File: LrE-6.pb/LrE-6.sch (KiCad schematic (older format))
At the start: 115 parts, among them J1 USB_B_Micro, J2 SM06B-SRSS-TB, J3 LP_Header_02x03, J4 LP_Header_01x02, Q1 2N7002, Q11 2N7002, SW1 SW_Push_45deg, SW10 SW_Push_45deg, SW11 Rotary_Encoder_Switch, SW12 Rotary_Encoder_Switch, SW13 Rotary_Encoder_Switch, SW14 Rotary_Encoder_Switch, SW15 Rotary_Encoder_Switch, SW16 Rotary_Encoder_Switch, SW2 SW_Push_45deg, SW3 SW_Push_45deg, SW4 SW_Push_45deg, SW5 SW_Push_45deg, SW6 SW_Push_45deg, SW7 SW_Push_45deg, SW8 SW_Push_45deg, SW9 SW_Push_45deg, U1 STM32F072C8Tx, U2 ESP-WROOM-02, U3 AQM0802-FLW-GBW, U4 SPX3819M5-L3-3TR

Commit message: 0.27-5
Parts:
- removed C20: 0.1u, Capacitor_SMD:C_0805_2012Metric, symbol LrE-6-rescue:C-Device
- removed C28: 10u, Capacitor_SMD:C_0805_2012Metric, symbol LrE-6-rescue:C-Device
- removed J3: LP_Header_02x03, Connector_PinHeader_2.54mm:PinHeader_2x03_P2.54mm_Vertical, symbol LrE-6-rescue:Conn_02x03_Odd_Even-Connector_Generic
- removed J4: LP_Header_01x02, Connector_PinHeader_2.54mm:PinHeader_1x02_P2.54mm_Vertical, symbol LrE-6-rescue:Conn_02x01-Connector_Generic
- removed R33: 10K, Resistor_SMD:R_0805_2012Metric, symbol LrE-6-rescue:R-Device
- removed R34: 100, Resistor_SMD:R_0805_2012Metric, symbol LrE-6-rescue:R-Device
- removed R36, R37: 10K, Resistor_SMD:R_0805_2012Metric, symbol Device:R
- removed U2: ESP-WROOM-02, RF_Module:ESP-WROOM-02, symbol LrE-6-rescue:ESP-WROOM-02-RF_Module
- C30, C31, C32, C33, C34, C35, C36: symbol Device:C -> LrE-6-rescue:C-Device
- Q1: symbol Transistor_FET:2N7002 -> LrE-6-rescue:2N7002-Transistor_FET
- R21: symbol Device:R -> LrE-6-rescue:R-Device
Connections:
- net labels removed: ENC6-A, ENC6-B, STM_RX, STM_TX, WL_0, WL_EN, WL_RST, WL_RXD, WL_TXD
- wire segments 462 -> 419
- no-connect marks 19 -> 14
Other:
- note added: "R2.1\n"
- note removed: "FT234X"
- note removed: "GND"
- note removed: "N.C.(5V)"
- note removed: "R2.02"
- note removed: "RXD"
- note removed: "TXD"
- moved on the sheet: Q1, R21

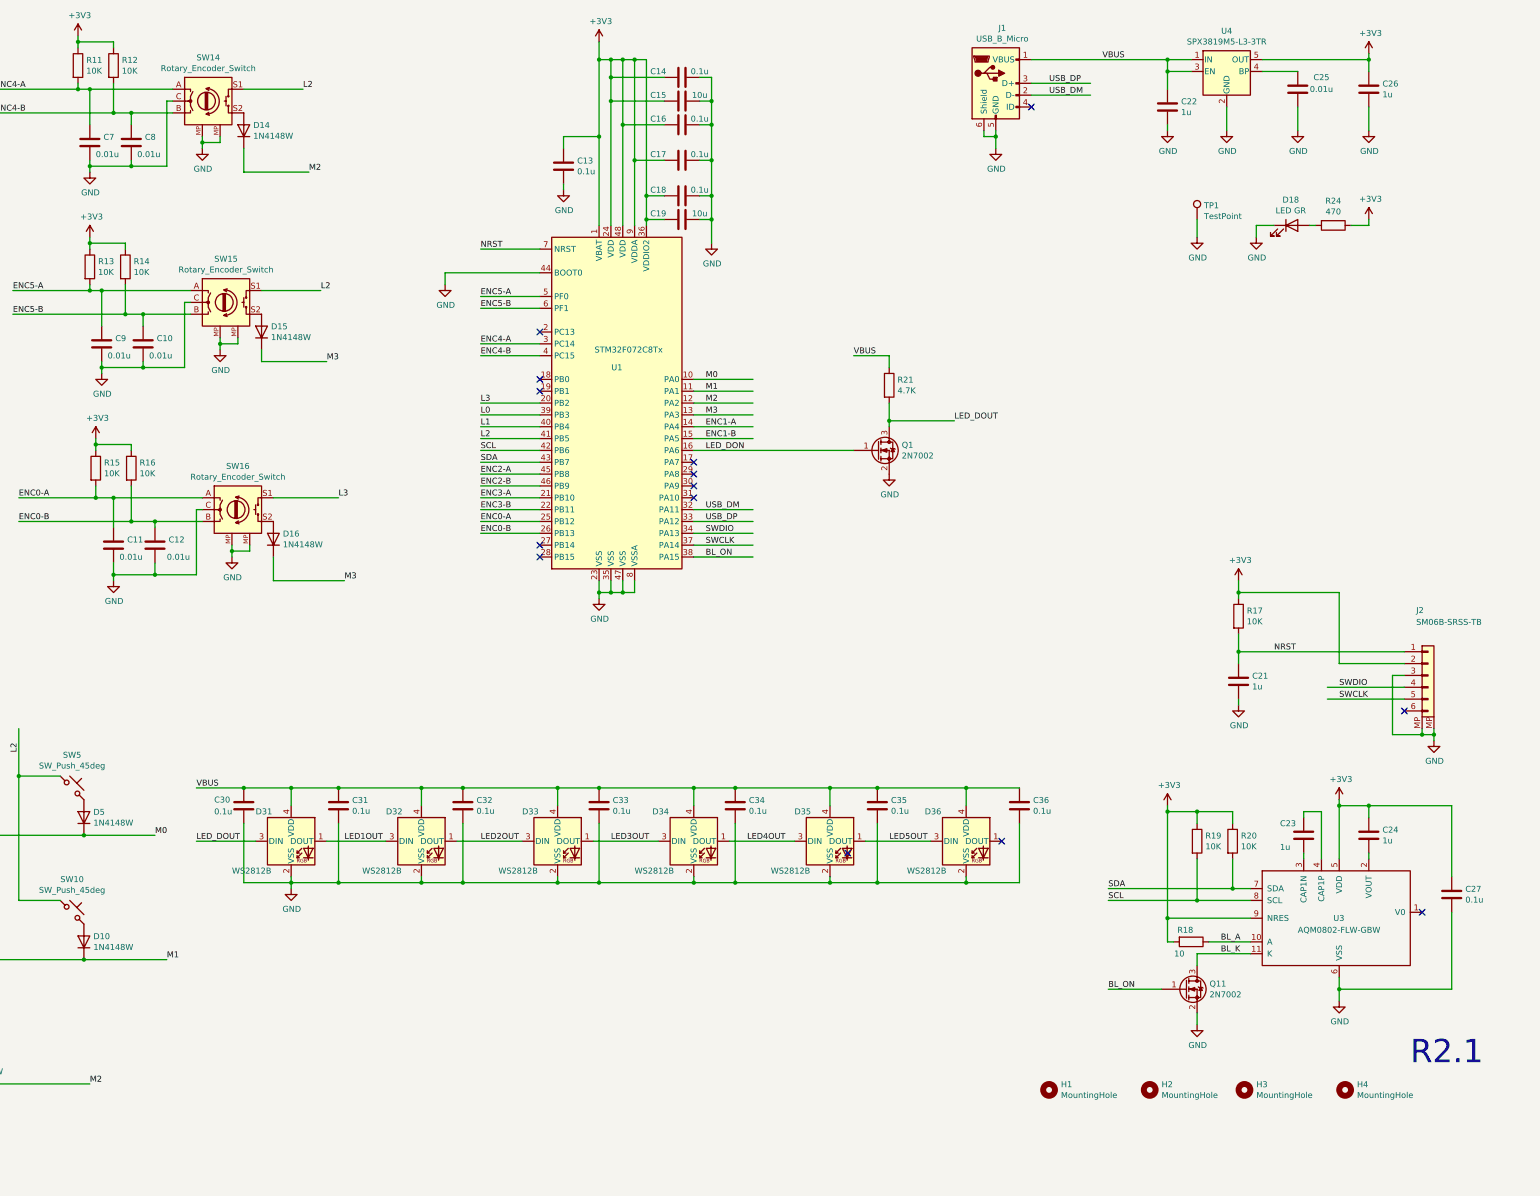
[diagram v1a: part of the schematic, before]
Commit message: pb R2.1pre
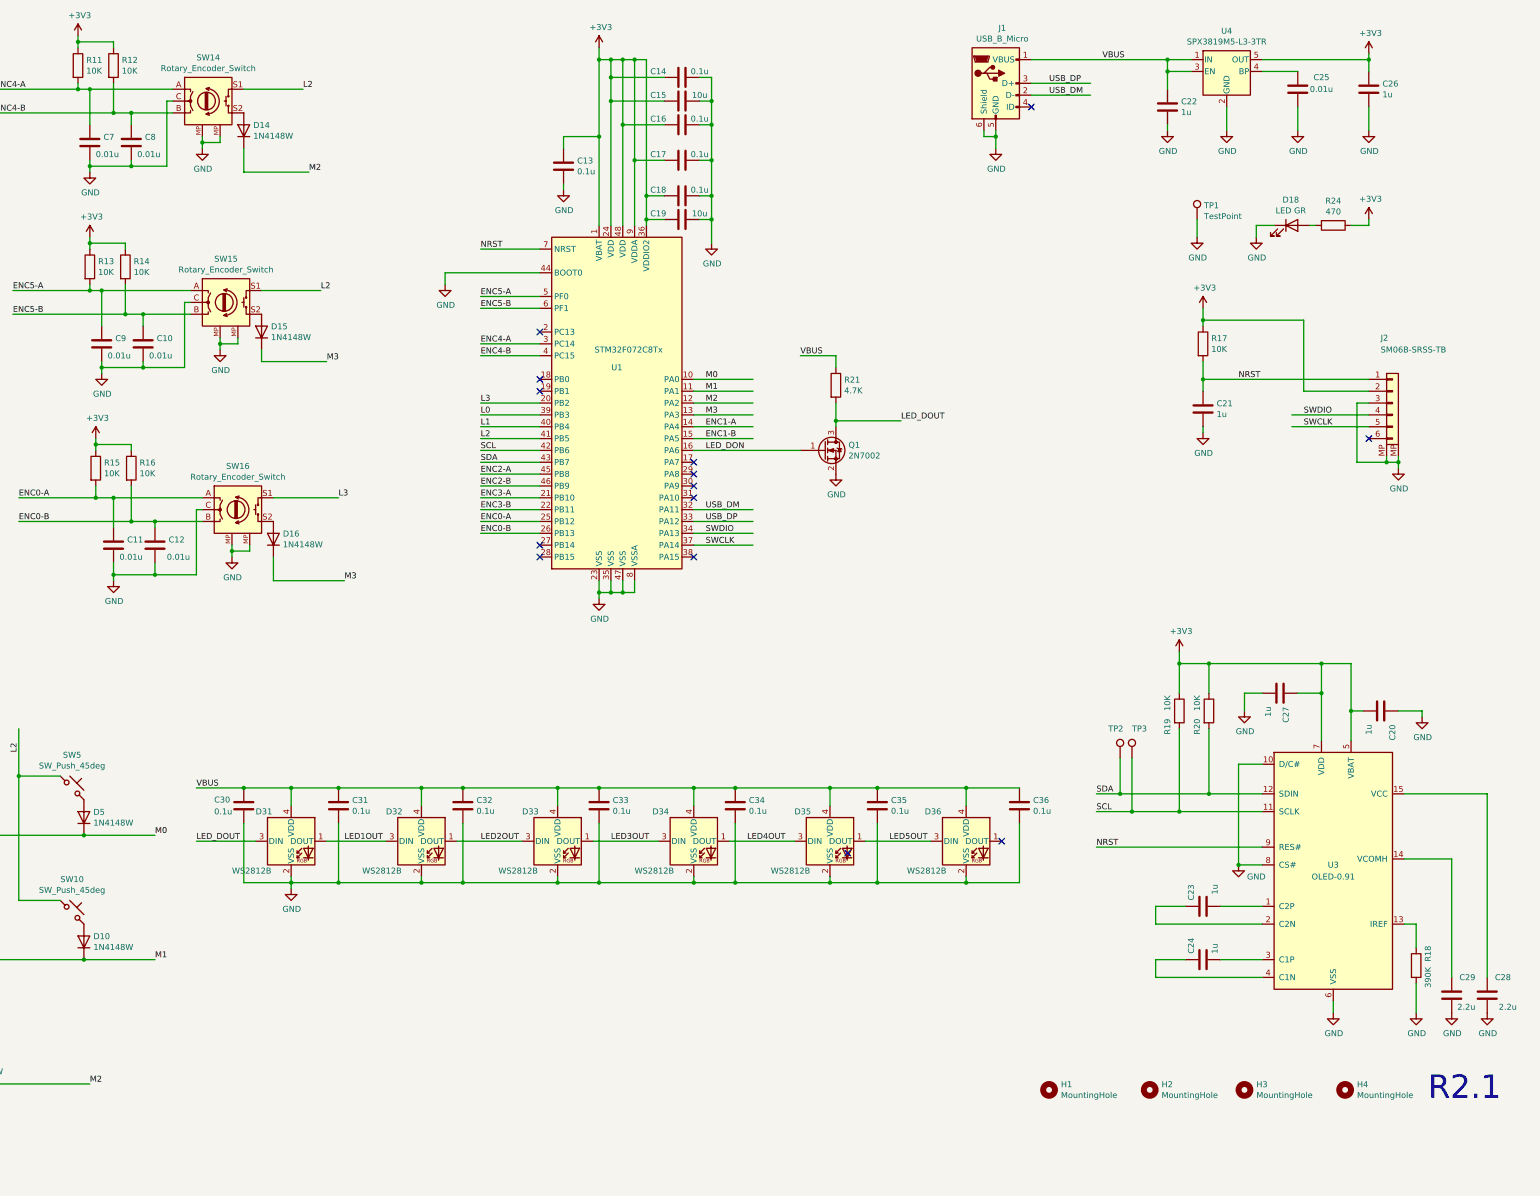
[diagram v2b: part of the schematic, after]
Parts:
- removed Q11: 2N7002, Package_TO_SOT_SMD:SOT-23, symbol LrE-6-rescue:2N7002-Transistor_FET
- removed U3: AQM0802-FLW-GBW, LrE-6:AQM0802_1, symbol LrE-6-rescue:AQM-LrE-6
- added C20: 1u, Capacitor_SMD:C_0805_2012Metric, symbol LrE-6-rescue:C-Device
- added C28, C29: 2.2u, Capacitor_SMD:C_0805_2012Metric, symbol LrE-6-rescue:C-Device
- added TP2, TP3: TestPoint-Connector, TestPoint:TestPoint_THTPad_D2.0mm_Drill1.0mm, symbol LrE-6-rescue:TestPoint-Connector
- added U3: OLED-0.91, LrE-6:OLED-9.1, symbol LrE-6:OLED-0.91
- C23, C24: footprint Capacitor_SMD:C_0603_1608Metric -> Capacitor_SMD:C_0805_2012Metric
- C27: value 0.1u -> 1u; footprint Capacitor_SMD:C_0603_1608Metric -> Capacitor_SMD:C_0805_2012Metric
- R18: value 10 -> 390K
- R19, R20: footprint Resistor_SMD:R_0805_2012Metric -> Resistor_SMD:R_0603_1608Metric
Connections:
- net labels removed: BL_A, BL_K, BL_ON
- wire segments 419 -> 429
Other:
- moved on the sheet: C21, C23, C24, C27, J2, Q1, R17, R18, R19, R20, R21

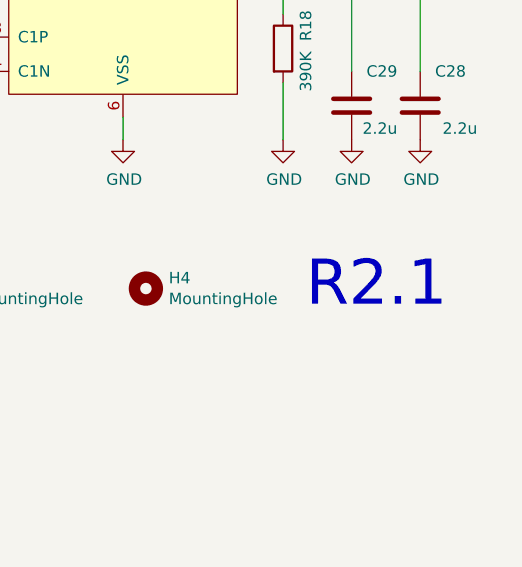
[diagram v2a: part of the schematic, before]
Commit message: 0.28-3
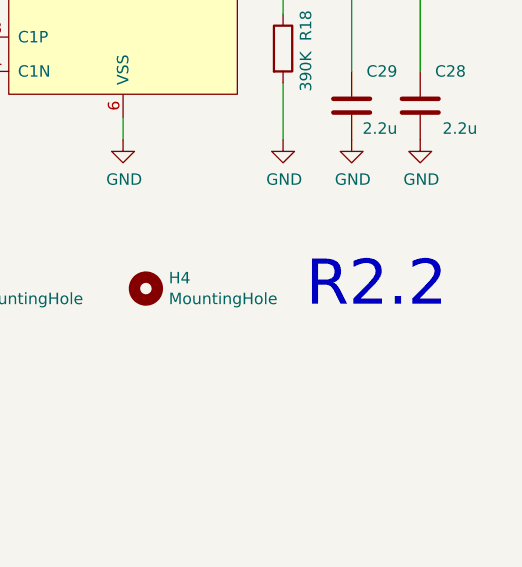
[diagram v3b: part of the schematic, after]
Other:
- note added: "R2.2\n"
- note removed: "R2.1\n"
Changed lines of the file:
@@
 	11650 1700 11650 1650
 Text Notes 15300 9850 0    197  ~ 0
-R2.1\n
+R2.2\n
 Wire Wire Line
 	1200 10900 1700 10900
